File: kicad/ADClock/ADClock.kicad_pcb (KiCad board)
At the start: 2 copper layers, 140 x 70 mm, 26 parts, among them IC1 ATMEGA328-PU, IC2 ATMEGA328-PU, Y1 Crystal, Y2 Crystal

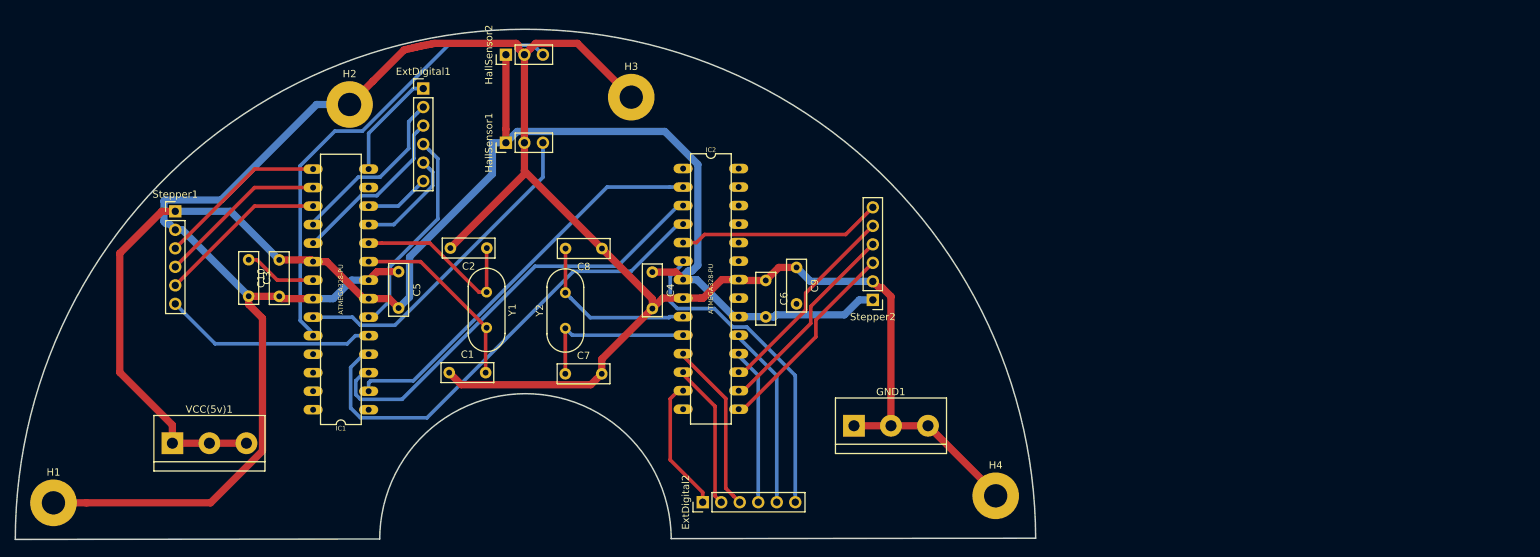
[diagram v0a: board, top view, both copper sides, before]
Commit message: board changes
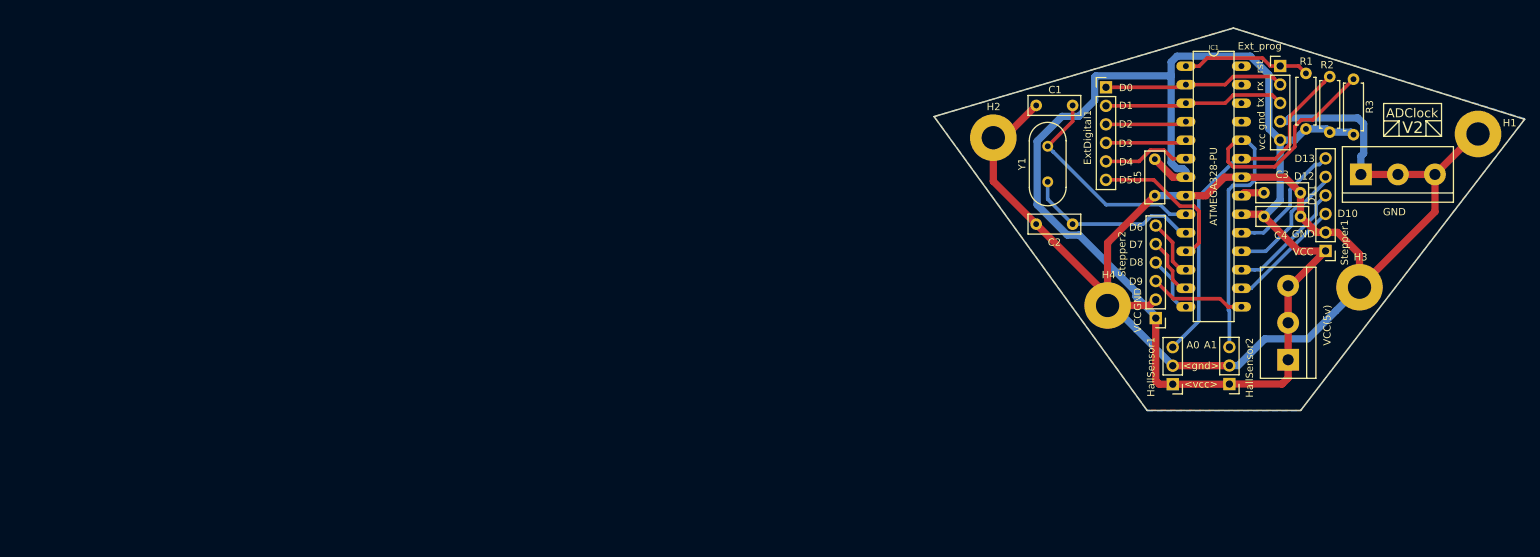
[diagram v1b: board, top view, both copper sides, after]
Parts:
- removed C10, C6, C7, C8, C9: C, Capacitor_THT:C_Rect_L7.0mm_W2.5mm_P5.00mm
- removed ExtDigital2: Conn_Ext_digital_2, Connector_PinHeader_2.54mm:PinHeader_1x06_P2.54mm_Vertical
- removed GND1: Screw_GND, TerminalBlock:TerminalBlock_bornier-3_P5.08mm
- removed IC2: ATMEGA328-PU, DIL28
- removed VCC(5v)1: Screw_VCC, TerminalBlock:TerminalBlock_bornier-3_P5.08mm
- removed Y2: Crystal, Crystal:Crystal_HC49-4H_Vertical
- added Ext_prog: Conn_Programmer, Connector_PinHeader_2.54mm:PinHeader_1x05_P2.54mm_Vertical, F.Cu at (200.1, 46.6)
- added GND: Screw_GND, TerminalBlock:TerminalBlock_bornier-3_P5.08mm, F.Cu at (211.2, 61.5)
- added R1: R, Resistor_THT:R_Axial_DIN0207_L6.3mm_D2.5mm_P7.62mm_Horizontal, F.Cu at (203.6, 47.6)
- added R2: R, Resistor_THT:R_Axial_DIN0207_L6.3mm_D2.5mm_P7.62mm_Horizontal, F.Cu at (206.9, 55.7)
- added R3: R, Resistor_THT:R_Axial_DIN0207_L6.3mm_D2.5mm_P7.62mm_Horizontal, F.Cu at (210.1, 56.0)
- added VCC(5v): Screw_VCC, TerminalBlock:TerminalBlock_bornier-3_P5.08mm, F.Cu at (201.2, 86.9)
- moved H1 201.9 mm to (227.2, 55.9)
- moved Stepper1 157.9 mm to (206.3, 72.0), turned to 180 degrees
- moved C3 139.6 mm to (197.9, 64.0), turned to 0 degrees
- moved IC1 120.6 mm to (191.0, 63.1), turned to 0 degrees
- moved HallSensor2 109.1 mm to (193.1, 90.3), turned to 180 degrees
- moved C5 104.3 mm to (182.9, 64.4), turned to 90 degrees
- moved H3 103.3 mm to (211.0, 77.0)
- moved HallSensor1 97.3 mm to (185.3, 90.3), turned to 180 degrees
- moved ExtDigital1 93.7 mm to (176.2, 49.5)
- moved C1 88.5 mm to (166.6, 52.0)
- moved H2 88.4 mm to (160.7, 56.4)
- moved C4 84.3 mm to (197.9, 67.3), turned to 0 degrees
- moved C2 80.4 mm to (171.6, 68.3)
- moved Y1 78.5 mm to (168.2, 62.5), turned to 90 degrees
- moved Stepper2 38.9 mm to (183.0, 81.2)
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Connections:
- IC1 pad 11: Net-(ExtDigital1-Pad5) -> Net-(ExtDigital1-Pad6)
- IC1 pad 12: Net-(ExtDigital1-Pad6) -> Net-(IC1-Pad12)
- IC1 pad 14: Net-(ExtDigital1-Pad1) -> Net-(IC1-Pad14)
- IC1 pad 18: Net-(ExtDigital1-Pad2) -> Net-(IC1-Pad18)
- IC1 pad 19: Net-(ExtDigital1-Pad3) -> Net-(IC1-Pad19)
- IC1 pad 2: Net-(IC1-Pad2) -> Net-(ExtDigital1-Pad1)
- IC1 pad 3: Net-(IC1-Pad3) -> Net-(ExtDigital1-Pad2)
- IC1 pad 4: Net-(IC1-Pad4) -> Net-(ExtDigital1-Pad3)
- IC1 pad 5: Net-(IC1-Pad5) -> Net-(ExtDigital1-Pad4)
- IC1 pad 6: Net-(ExtDigital1-Pad4) -> Net-(ExtDigital1-Pad5)
- Stepper1 pad 3: Net-(IC1-Pad15) -> Net-(IC1-Pad16)
- Stepper1 pad 4: Net-(IC1-Pad16) -> Net-(IC1-Pad17)
- Stepper1 pad 5: Net-(IC1-Pad17) -> Net-(IC1-Pad18)
- Stepper1 pad 6: Net-(IC1-Pad5) -> Net-(IC1-Pad19)
- Stepper2 pad 3: Net-(IC2-Pad15) -> Net-(IC1-Pad15)
- Stepper2 pad 4: Net-(IC2-Pad16) -> Net-(IC1-Pad14)
- Stepper2 pad 5: Net-(IC2-Pad17) -> Net-(IC1-Pad13)
- Stepper2 pad 6: Net-(IC2-Pad5) -> Net-(IC1-Pad12)
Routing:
- net Net-(C1-Pad1): track 341.1 -> 201.6 mm
- net Net-(IC1-Pad4): track 66.0 -> 0.00 mm
- net Net-(IC1-Pad3): track 60.3 -> 0.00 mm
- net Net-(IC1-Pad2): track 55.4 -> 0.00 mm
- net Net-(ExtDigital2-Pad6): track 45.0 -> 0.00 mm
- net Net-(IC1-Pad5): track 29.3 -> 0.00 mm
- net Net-(IC2-Pad16): track 28.1 -> 0.00 mm
- net Net-(IC2-Pad17): track 28.1 -> 0.00 mm
- net Net-(IC2-Pad15): track 28.1 -> 0.00 mm
- net Net-(IC2-Pad5): track 28.0 -> 0.00 mm
- net Net-(ExtDigital2-Pad5): track 25.1 -> 0.00 mm
- net Net-(C8-Pad2): track 23.7 -> 0.00 mm
- net Net-(ExtDigital2-Pad3): track 23.6 -> 0.00 mm
- net Net-(C7-Pad1): track 22.8 -> 0.00 mm
- net Net-(ExtDigital2-Pad4): track 21.5 -> 0.00 mm
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- added copper zone on B.Cu, net Net-(C1-Pad1)
- added copper zone on F.Cu, net Net-(C1-Pad1)
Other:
- board size 140 x 70 mm -> 81 x 52.5 mm
- board text added: "<gnd>"
- board text added: "<vcc>"
- board text added: "A0"
- board text added: "A1"
- board text added: "ADClock"
- board text added: "D0"
- board text added: "D1"
- board text added: "D10"
- board text added: "D11"
- board text added: "D12"
- board text added: "D13"
- board text added: "D2"
- board text added: "D3"
- board text added: "D4"
- board text added: "D5"
- board text added: "D6"
- board text added: "D7"
- board text added: "D8"
- board text added: "D9"
- board text added: "GND"
- board text added: "V2"
- board text added: "VCC"
- board text added: "gnd"
- board text added: "rst"
- board text added: "rx"
- board text added: "tx"
- board text added: "vcc"
